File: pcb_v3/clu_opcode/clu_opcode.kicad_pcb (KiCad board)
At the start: 2 copper layers, 10.2 x 113 mm, 44 parts, among them J2 Conn_01x09, J3 Conn_01x09

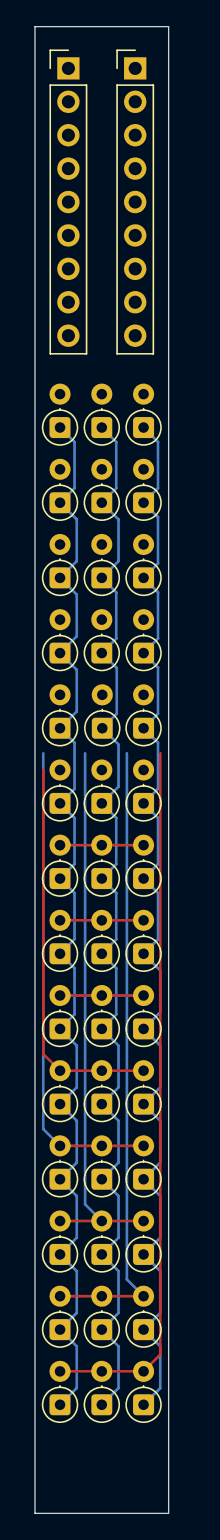
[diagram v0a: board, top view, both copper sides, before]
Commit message: .
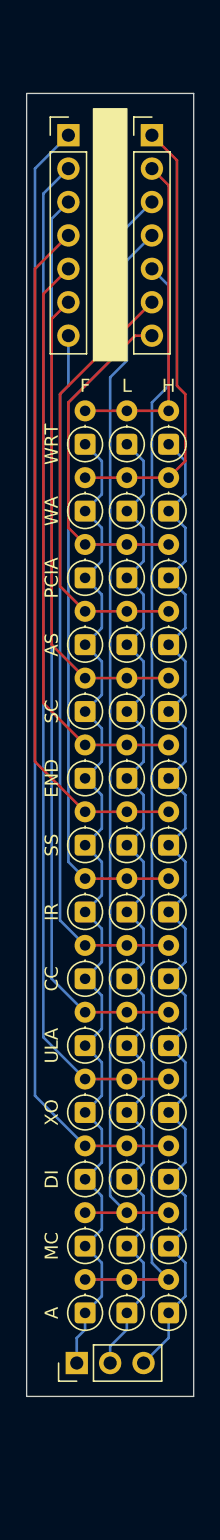
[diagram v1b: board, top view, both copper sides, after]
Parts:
- added J1: Conn_01x07, Connector_PinHeader_2.54mm:PinHeader_1x07_P2.54mm_Vertical, F.Cu at (64.8, 49.5)
- J2: value Conn_01x09 -> Conn_01x07; footprint Connector_PinHeader_2.54mm:PinHeader_1x09_P2.54mm_Vertical -> Connector_PinHeader_2.54mm:PinHeader_1x07_P2.54mm_Vertical
- J3: value Conn_01x09 -> Conn_01x03; footprint Connector_PinHeader_2.54mm:PinHeader_1x09_P2.54mm_Vertical -> Connector_PinHeader_2.54mm:PinHeader_1x03_P2.54mm_Vertical
- moved J3 98.5 mm to (65.4, 142.9), turned to 90 degrees
- moved J2 8.13 mm to (71.1, 49.5)
- moved D40 7.24 mm to (66.0, 139.1)
- moved D41 7.24 mm to (69.2, 139.1)
- moved D42 7.24 mm to (72.4, 139.1)
- moved D37 6.63 mm to (66.0, 134.0)
- moved D38 6.63 mm to (69.2, 134.0)
- moved D39 6.63 mm to (72.4, 134.0)
- moved D34 6.02 mm to (66.0, 128.9)
- moved D35 6.02 mm to (69.2, 128.9)
- moved D36 6.02 mm to (72.4, 128.9)
- moved D31 5.43 mm to (66.0, 123.8)
- moved D32 5.43 mm to (69.2, 123.8)
- moved D33 5.43 mm to (72.4, 123.8)
- moved D28 4.84 mm to (66.0, 118.7)
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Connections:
- J2 pad 1: ~{fetch_cycle} -> ~{UC_write_address}
- J2 pad 2: ~{low_cycle} -> ~{UC_write_enable}
- J2 pad 3: ~{high_cycle} -> ~{UC_int_ready}
- J2 pad 4: ~{UC_write_enable} -> ~{UC_read_mem_const}
- J2 pad 5: ~{UC_write_address} -> ~{UC_A}
- J2 pad 6: ~{UC_pcia_swap} -> ~{UC_read_addr_src_reg}
- J2 pad 7: ~{UC_read_addr_src_reg} -> ~{UC_pcia_swap}
- J3 pad 1: ~{UC_save_src_reg} -> ~{fetch_cycle}
- J3 pad 2: ~{UC_int_ready} -> ~{low_cycle}
- J3 pad 3: ~{UC_clear_cond_reg} -> ~{high_cycle}
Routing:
- net ~{UC_int_ready}: track 6.35 -> 60.9 mm
- net ~{UC_clear_cond_reg}: track 6.35 -> 53.8 mm
- net ~{UC_save_src_reg}: track 6.35 -> 52.8 mm
- net ~{UC_restart_cycle}: track 0.00 -> 44.6 mm
- net ~{UC_disable_int}: track 42.4 -> 85.8 mm
- net ~{UC_extended_opcode}: track 36.7 -> 77.7 mm
- net ~{UC_ula_enable}: track 29.7 -> 69.5 mm
- net ~{UC_save_cond_reg}: track 0.00 -> 36.5 mm
- net ~{UC_read_mem_const}: track 48.2 -> 82.5 mm
- net ~{UC_write_address}: track 0.00 -> 34.0 mm
- net ~{UC_read_addr_src_reg}: track 0.00 -> 33.5 mm
- net ~{UC_A}: track 53.9 -> 84.8 mm
- net ~{UC_pcia_swap}: track 0.00 -> 26.1 mm
- net ~{UC_write_enable}: track 0.00 -> 25.3 mm
- net ~{fetch_cycle}: track 87.3 -> 83.8 mm
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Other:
- board size 10.2 x 113 mm -> 12.7 x 99.1 mm
- board text added: "A"
- board text added: "AS"
- board text added: "CC"
- board text added: "DI"
- board text added: "END"
- board text added: "F"
- board text added: "H"
- board text added: "IR"
- board text added: "L"
- board text added: "MC"
- board text added: "PCIA"
- board text added: "SC"
- board text added: "SS"
- board text added: "ULA"
- board text added: "WA"
- board text added: "WRT"
- board text added: "XO"
